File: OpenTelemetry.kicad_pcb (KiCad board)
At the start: 2 copper layers, 142.2 x 73.7 mm, 23 parts, among them J1 Conn_ARM_JTAG_SWD_10, J2 Conn_01x09, J3 USB_B_Micro, U1 Adafruit-GPS, U2 TCAN1042xV, U3 STM32F072RBTx, U4 Adafruit-BNO055, U5 RFD900x, U6 HY28B

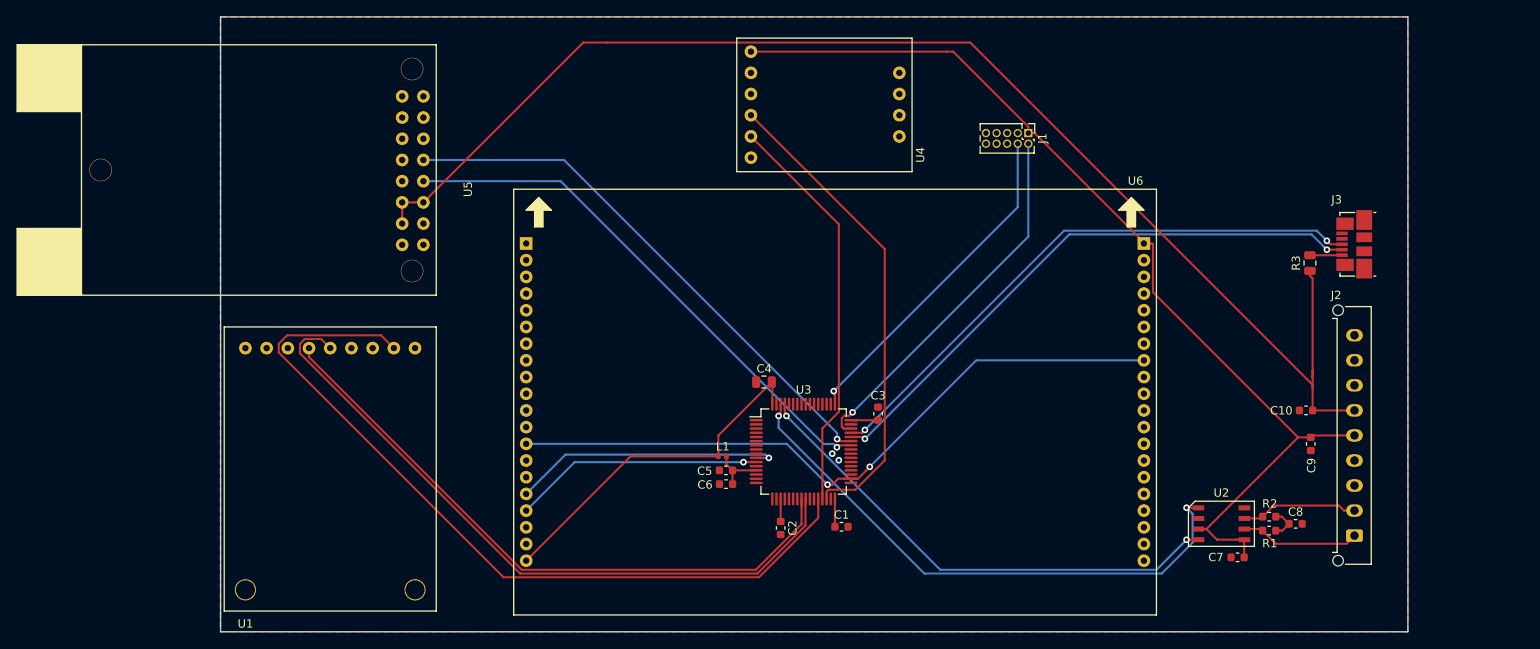
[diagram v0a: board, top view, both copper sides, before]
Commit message: V1 finished
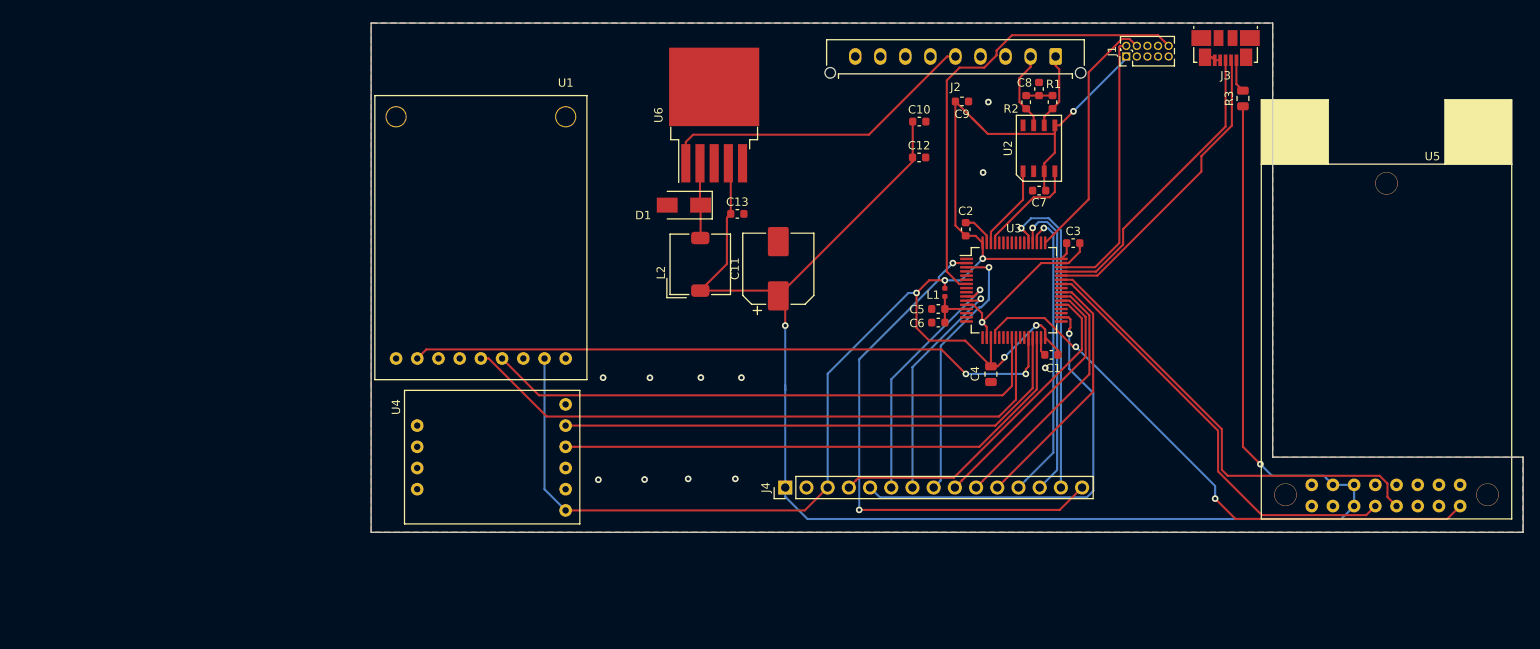
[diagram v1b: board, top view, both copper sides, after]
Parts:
- added C11: 220uF, Capacitor_SMD:CP_Elec_8x10, F.Cu at (127.8, 78.4)
- added C12: 100nF, Capacitor_SMD:C_0603_1608Metric, F.Cu at (144.6, 65.1)
- added C13: 100nF, Capacitor_SMD:C_0603_1608Metric, F.Cu at (122.9, 71.9)
- added D1: D_Schottky, Diode_SMD:D_SMA, F.Cu at (116.5, 70.8)
- added J4: Conn_01x15_Female, Connector_PinHeader_2.54mm:PinHeader_1x15_P2.54mm_Vertical, F.Cu at (128.6, 104.6)
- added L2: 33uH, Inductor_SMD:L_TDK_SLF7045, F.Cu at (118.4, 77.9)
- U6: value HY28B -> LM2596S-5; footprint JohnLib:HY28B -> Package_TO_SOT_SMD:TO-263-5_TabPin3
- moved U5 102.4 mm to (185.6, 108.4), turned to 0 degrees
- moved J2 67.6 mm to (161.0, 53.0), turned to 180 degrees
- moved U4 61.2 mm to (104.0, 109.0), turned to 90 degrees
- moved C8 60.5 mm to (159.0, 56.9), turned to 90 degrees
- moved C9 58.6 mm to (149.8, 58.4), turned to 0 degrees
- moved C10 57.8 mm to (144.7, 60.8), turned to 0 degrees
- moved R2 57.6 mm to (157.5, 58.5), turned to 90 degrees
- moved R1 57.5 mm to (160.6, 58.5), turned to 90 degrees
- moved U2 50.0 mm to (159.0, 64.0), turned to 0 degrees
- moved C7 49.9 mm to (159.0, 69.1)
- moved C2 42.1 mm to (150.2, 73.7), turned to 90 degrees
- moved L1 33.1 mm to (147.7, 81.3), turned to 90 degrees
- moved C1 32.5 mm to (160.5, 88.7), turned to 180 degrees
- moved C6 32.0 mm to (146.9, 84.9)
- moved C5 32.0 mm to (146.9, 83.2)
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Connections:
- net /MISO renamed Net-(U3-Pad56)
- net /MOSI renamed Net-(U3-Pad57)
- net /SCK renamed Net-(U3-Pad55)
- J2 pad 4: Net-(J2-Pad4) -> GND
- J2 pad 5: +3V3 -> /Batt+
- J2 pad 6: +5V -> Net-(J2-Pad6)
- U3 pad 2: Net-(U3-Pad2) -> /TP_X+
- U3 pad 3: Net-(U3-Pad3) -> /LCD_CS
- U3 pad 37: Net-(U3-Pad37) -> /LITE
- U3 pad 38: Net-(U3-Pad38) -> /LCD_RST
- U3 pad 39: Net-(U3-Pad39) -> /LCD_WAIT
- U3 pad 40: Net-(U3-Pad40) -> /LCD_INT
- U3 pad 51: Net-(U3-Pad51) -> /TP_Y+
- U3 pad 52: Net-(U3-Pad52) -> /TP_Y-
- U3 pad 53: Net-(U3-Pad53) -> /TP_X-
- U6 pad 1: Net-(U6-Pad1) -> /Batt+
- U6 pad 2: GND -> /Reg_Out
- U6 pad 4: GND -> +5V
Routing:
- net /GPIO_1: track 0.00 -> 68.7 mm, vias 0 -> 2
- net /TP_X+: track 0.00 -> 63.7 mm, vias 0 -> 2
- net /TXD: track 67.2 -> 10.2 mm, vias 2 -> 0
- net /NRST: track 0.00 -> 55.6 mm
- net +5V: track 159.5 -> 207.4 mm, vias 0 -> 2
- net /RXD: track 60.0 -> 12.6 mm, vias 2 -> 0
- net /LITE: track 0.00 -> 41.6 mm
- net /Batt+: track 0.00 -> 39.1 mm
- net /TP_X-: track 0.00 -> 38.8 mm, vias 0 -> 1
- net /TP_Y-: track 0.00 -> 37.0 mm, vias 0 -> 1
- net /TP_Y+: track 0.00 -> 35.7 mm, vias 0 -> 1
- net /USB+: track 69.5 -> 35.9 mm, vias 2 -> 0
- net /USB-: track 69.8 -> 36.8 mm, vias 2 -> 0
- net /LCD_CS: track 0.00 -> 32.0 mm, vias 0 -> 1
- net /LCD_SCK: track 82.2 -> 50.6 mm, vias 2 -> 1
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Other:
- board size 142.2 x 73.7 mm -> 138 x 61 mm
